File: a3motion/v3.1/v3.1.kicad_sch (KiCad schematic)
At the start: 0 parts

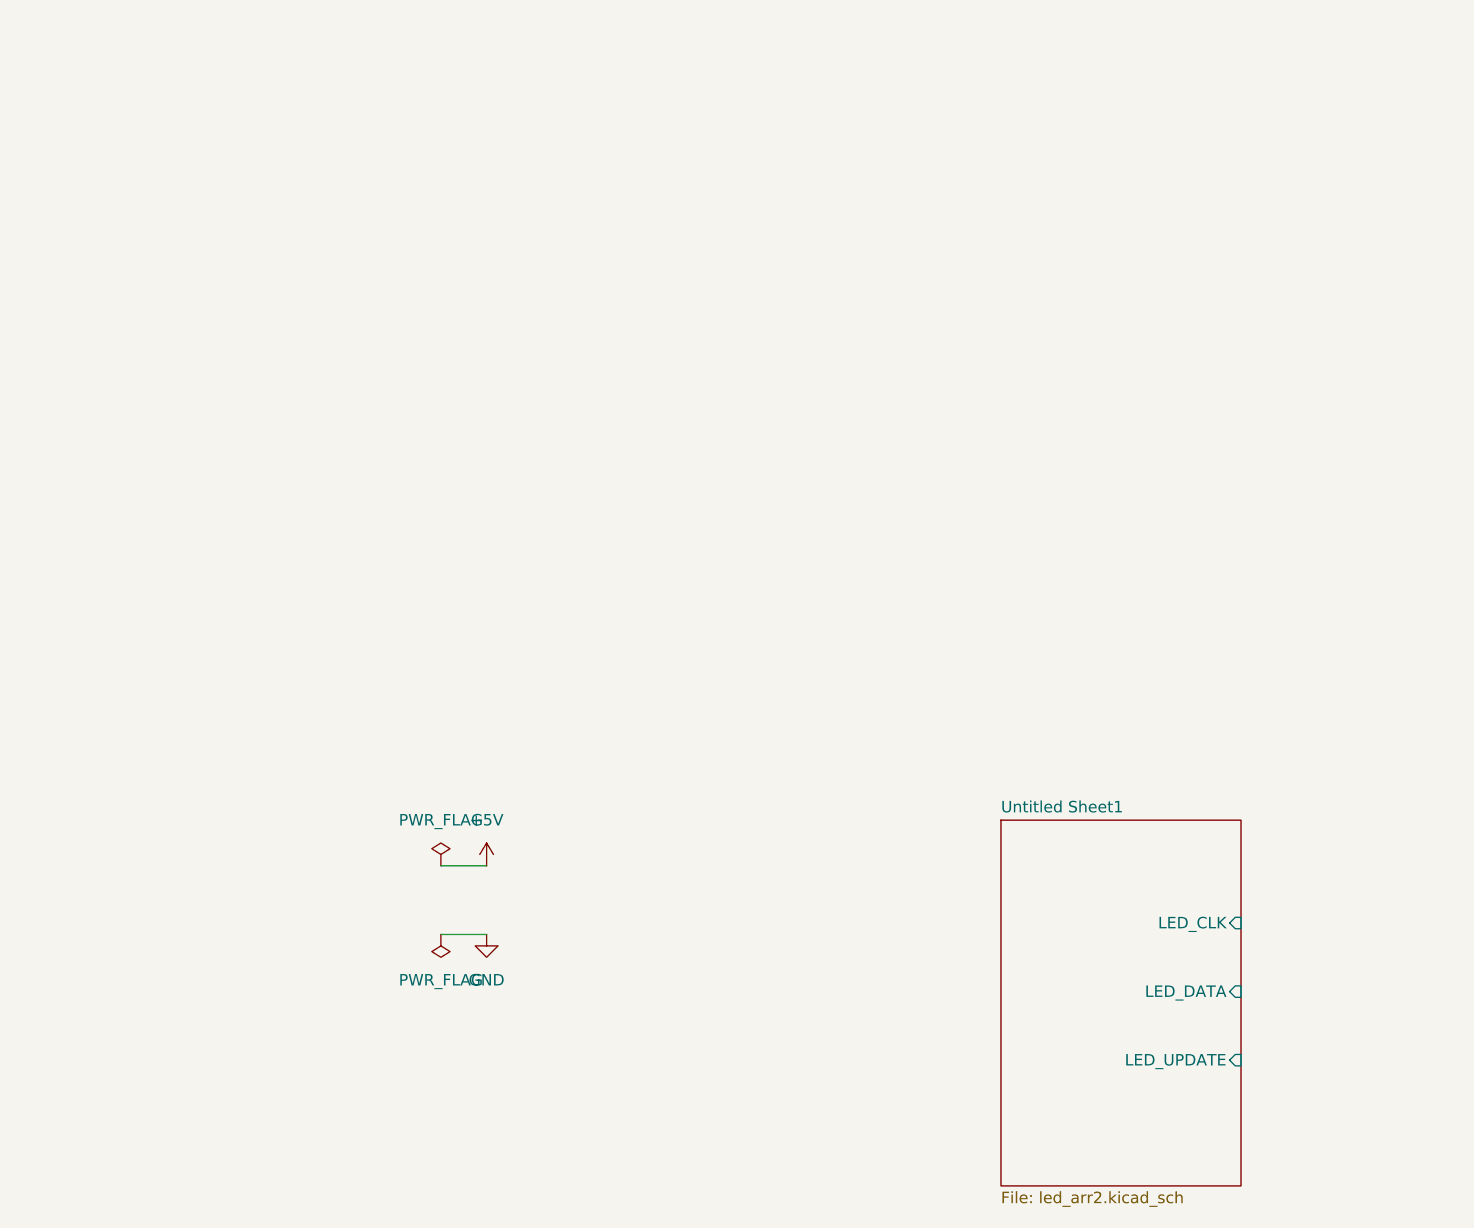
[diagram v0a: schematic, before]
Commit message: .
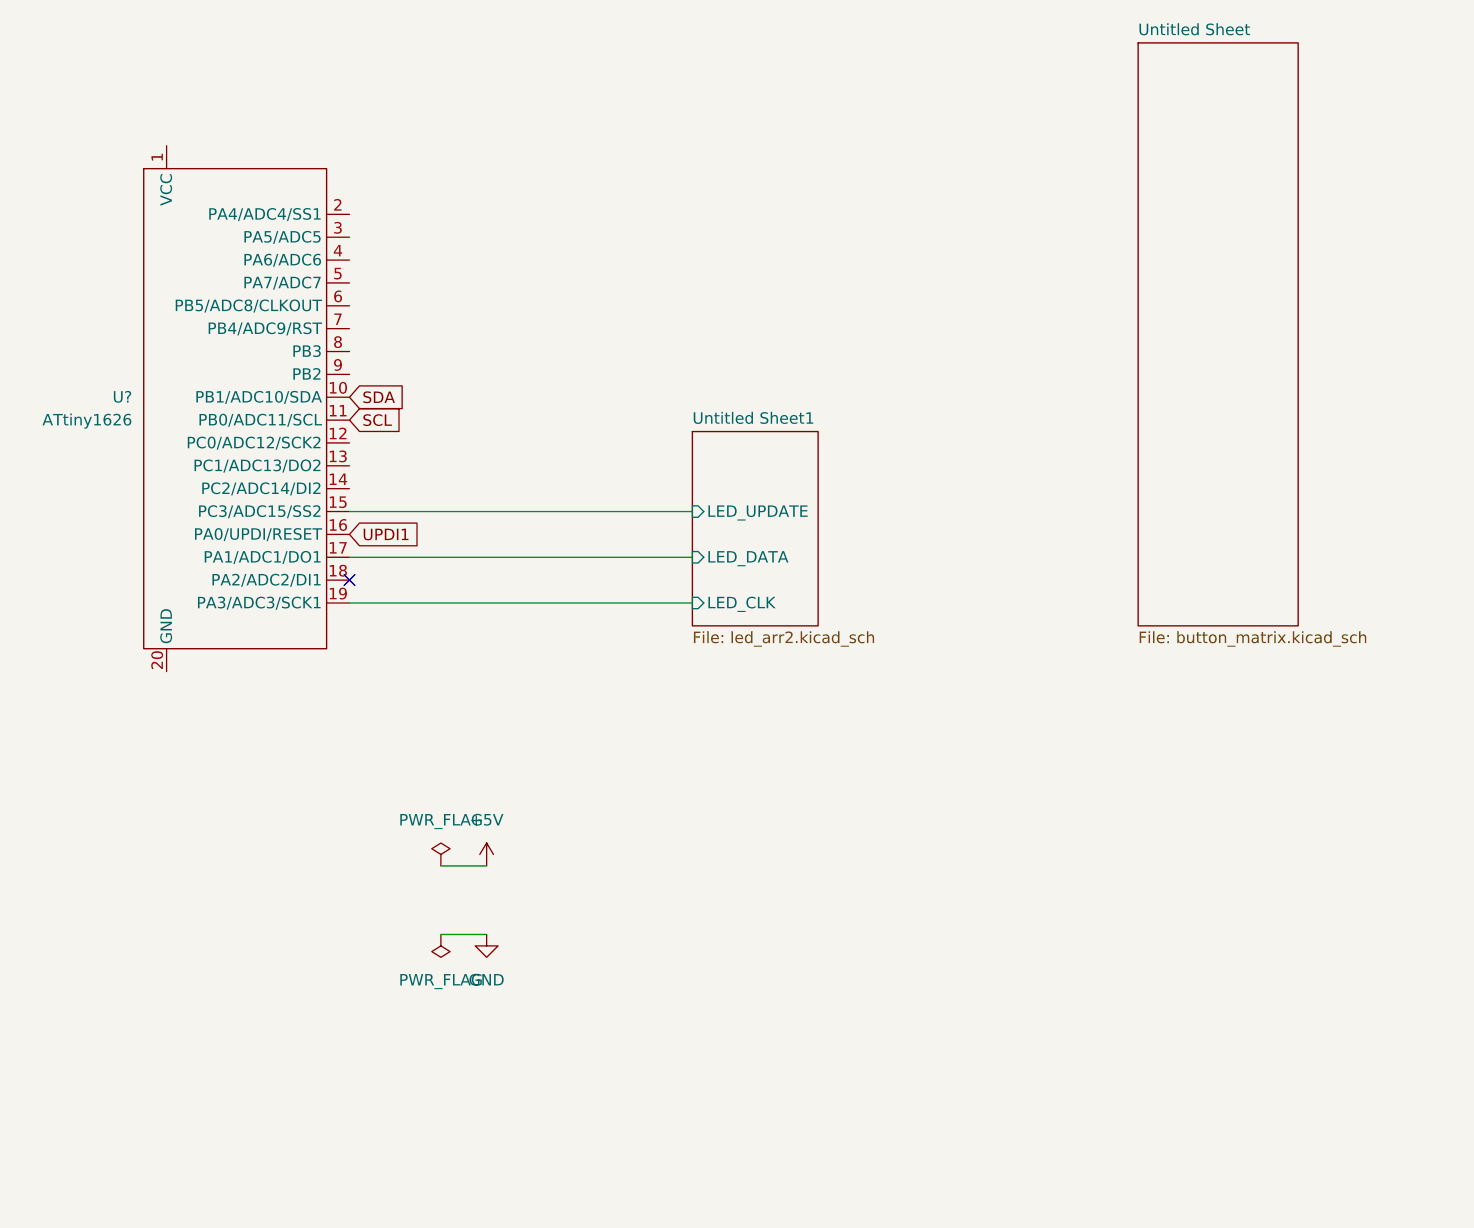
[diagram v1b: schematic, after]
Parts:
- added U?: ATtiny1626, attiny1626:SOIC127P1030X265-20N, symbol 3dAudioSym:ATtiny1626
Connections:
- net Untitled Sheet1/LED_CLK: now also U?.19 (PA3/ADC3/SCK1)
- net Untitled Sheet1/LED_DATA: now also U?.17 (PA1/ADC1/DO1)
- net Untitled Sheet1/LED_UPDATE: now also U?.15 (PC3/ADC15/SS2)
- new net SCL: U?.11 (PB0/ADC11/SCL)
- new net SDA: U?.10 (PB1/ADC10/SDA)
- new net UPDI1: U?.16 (PA0/UPDI/RESET)
- no-connect marks 0 -> 1
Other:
- added sheet Untitled Sheet (button_matrix.kicad_sch)
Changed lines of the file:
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@@
 (kicad_sch (version 20211123) (generator eeschema)
   (paper "A4")
+  (no_connect (at 53.34 82.55))
   (wire (pts (xy 63.5 114.3) (xy 68.58 114.3))
     (stroke (width 0) (type default) (color 0 0 0 0))
@@
   (wire (pts (xy 63.5 121.92) (xy 68.58 121.92))
     (stroke (width 0) (type default) (color 0 0 0 0))
+  )
+  (wire (pts (xy 53.34 80.01) (xy 91.44 80.01))
+    (stroke (width 0) (type default) (color 0 0 0 0))
+  )
+  (wire (pts (xy 53.34 74.93) (xy 91.44 74.93))
+    (stroke (width 0) (type default) (color 0 0 0 0))
+  )
+  (wire (pts (xy 53.34 85.09) (xy 91.44 85.09))
+    (stroke (width 0) (type default) (color 0 0 0 0))
+  )
+  (global_label "SCL" (shape input) (at 53.34 64.77 0) (fields_autoplaced)
+    (effects (font (size 1.27 1.27)) (justify left))
+    (property "Intersheet References" "${INTERSHEET_REFS}" (id 0) (at 59.2607 64.6906 0)
+      (effects (font (size 1.27 1.27)) (justify left) hide)
+    )
+  )
+  (global_label "UPDI1" (shape input) (at 53.34 77.47 0) (fields_autoplaced)
+    (effects (font (size 1.27 1.27)) (justify left))
+    (property "Intersheet References" "${INTERSHEET_REFS}" (id 0) (at 61.4379 77.3906 0)
+      (effects (font (size 1.27 1.27)) (justify left) hide)
+    )
+  )
+  (global_label "SDA" (shape input) (at 53.34 62.23 0) (fields_autoplaced)
+    (effects (font (size 1.27 1.27)) (justify left))
+    (property "Intersheet References" "${INTERSHEET_REFS}" (id 0) (at 59.3212 62.1506 0)
+      (effects (font (size 1.27 1.27)) (justify left) hide)
+    )
   )
   (symbol (lib_id "power:PWR_FLAG") (at 63.5 121.92 180) (unit 1)
@@
     (pin "1")
   )
-  (sheet (at 125.73 109.22) (size 26.67 40.64) (fields_autoplaced)
+  (symbol (lib_id "3dAudioSym:ATtiny1626") (at 41.91 64.77 0) (unit 1)
+    (in_bom yes) (on_board yes) (fields_autoplaced)
+    (property "Reference" "U?" (id 0) (at 29.21 62.2299 0)
+      (effects (font (size 1.27 1.27)) (justify right))
+    )
+    (property "Value" "ATtiny1626" (id 1) (at 29.21 64.7699 0)
+      (effects (font (size 1.27 1.27)) (justify right))
+    )
+    (property "Footprint" "attiny1626:SOIC127P1030X265-20N" (id 2) (at 53.34 39.37 0)
+      (effects (font (size 1.27 1.27)) hide)
+    )
+    (property "Datasheet" "" (id 3) (at 53.34 39.37 0)
+      (effects (font (size 1.27 1.27)) hide)
+    )
+    (pin "1")
+    (pin "10")
+    (pin "11")
+    (pin "12")
+    (pin "13")
+    (pin "14")
+    (pin "15")
+    (pin "16")
+    (pin "17")
+    (pin "18")
+    (pin "19")
+    (pin "2")
+    (pin "20")
+    (pin "3")
+    (pin "4")
+    (pin "5")
+    (pin "6")
+    (pin "7")
+    (pin "8")
+    (pin "9")
+  )
+  (sheet (at 91.44 66.04) (size 13.97 21.59) (fields_autoplaced)
     (stroke (width 0.1524) (type solid) (color 0 0 0 0))
     (fill (color 0 0 0 0.0000))
-    (property "Sheet name" "Untitled Sheet1" (id 0) (at 125.73 108.5084 0)
+    (property "Sheet name" "Untitled Sheet1" (id 0) (at 91.44 65.3284 0)
       (effects (font (size 1.27 1.27)) (justify left bottom))
     )
-    (property "Sheet file" "led_arr2.kicad_sch" (id 1) (at 125.73 150.4446 0)
+    (property "Sheet file" "led_arr2.kicad_sch" (id 1) (at 91.44 88.2146 0)
       (effects (font (size 1.27 1.27)) (justify left top))
     )
-    (pin "LED_CLK" input (at 152.4 120.65 0)
-      (effects (font (size 1.27 1.27)) (justify right))
-    )
-    (pin "LED_DATA" input (at 152.4 128.27 0)
-      (effects (font (size 1.27 1.27)) (justify right))
-    )
-    (pin "LED_UPDATE" input (at 152.4 135.89 0)
-      (effects (font (size 1.27 1.27)) (justify right))
+    (pin "LED_CLK" input (at 91.44 85.09 180)
+      (effects (font (size 1.27 1.27)) (justify left))
+    )
+    (pin "LED_DATA" input (at 91.44 80.01 180)
+      (effects (font (size 1.27 1.27)) (justify left))
+    )
+    (pin "LED_UPDATE" input (at 91.44 74.93 180)
+      (effects (font (size 1.27 1.27)) (justify left))
+    )
+  )
+  (sheet (at 140.97 22.86) (size 17.78 64.77) (fields_autoplaced)
+    (stroke (width 0.1524) (type solid) (color 0 0 0 0))
+    (fill (color 0 0 0 0.0000))
+    (property "Sheet name" "Untitled Sheet" (id 0) (at 140.97 22.1484 0)
+      (effects (font (size 1.27 1.27)) (justify left bottom))
+    )
+    (property "Sheet file" "button_matrix.kicad_sch" (id 1) (at 140.97 88.2146 0)
+      (effects (font (size 1.27 1.27)) (justify left top))
     )
   )
@@
     (path "/" (page "1"))
     (path "/8485fc92-3a6c-45d4-b117-a7f692d410d2" (page "3"))
+    (path "/fc444129-c0ee-4f1d-b15d-2ca12b630041" (page "3"))
   )
   (symbol_instances
@@
       (reference "R59") (unit 1) (value "4K7") (footprint "Resistor_SMD:R_1206_3216Metric_Pad1.30x1.75mm_HandSolder")
     )
+    (path "/fc444129-c0ee-4f1d-b15d-2ca12b630041/24e5708f-47e8-44cb-a8f1-6278ec5740e5"
+      (reference "R?") (unit 1) (value "R") (footprint "")
+    )
+    (path "/fc444129-c0ee-4f1d-b15d-2ca12b630041/3942fb96-a42e-455d-bf11-cb4cfc9b1fbd"
+      (reference "R?") (unit 1) (value "R") (footprint "")
+    )
+    (path "/fc444129-c0ee-4f1d-b15d-2ca12b630041/5a28c5f0-590c-4954-8ba8-3af237537b52"
+      (reference "R?") (unit 1) (value "R") (footprint "")
+    )
+    (path "/fc444129-c0ee-4f1d-b15d-2ca12b630041/5b3a3957-e2a8-4c0e-b421-5c753ea740f5"
+      (reference "R?") (unit 1) (value "R") (footprint "")
+    )
+    (path "/fc444129-c0ee-4f1d-b15d-2ca12b630041/635bd6f6-0714-4edd-8cc0-90ff7d08cab1"
+      (reference "R?") (unit 1) (value "R") (footprint "")
+    )
+    (path "/fc444129-c0ee-4f1d-b15d-2ca12b630041/88b0357f-5c8c-4fca-a7c2-9c8e643ff511"
+      (reference "R?") (unit 1) (value "R") (footprint "")
+    )
+    (path "/fc444129-c0ee-4f1d-b15d-2ca12b630041/a5884584-137e-4379-a7f7-6c3f1c075971"
+      (reference "R?") (unit 1) (value "R") (footprint "")
+    )
+    (path "/fc444129-c0ee-4f1d-b15d-2ca12b630041/d2182e5f-de5f-4505-85f8-51877d61a915"
+      (reference "R?") (unit 1) (value "R") (footprint "")
+    )
     (path "/8485fc92-3a6c-45d4-b117-a7f692d410d2/dcc539c5-e251-4449-af3b-095764ed56b3"
       (reference "U1") (unit 1) (value "TPIC6C595") (footprint "Package_SO:SOIC-16_3.9x9.9mm_P1.27mm")
@@
       (reference "U6") (unit 1) (value "TPIC6C595") (footprint "Package_SO:SOIC-16_3.9x9.9mm_P1.27mm")
     )
-  )
+    (path "/fc444129-c0ee-4f1d-b15d-2ca12b630041/1dc51fd4-c2fb-4171-8240-bdbc958c22ae"
+      (reference "U?") (unit 1) (value "touch_but_square") (footprint "3dAudioFoot:But_Velo_Rec_1")
+    )
+    (path "/fc444129-c0ee-4f1d-b15d-2ca12b630041/3e13a1a2-ca0d-42b0-b43f-ba376b17b285"
+      (reference "U?") (unit 1) (value "touch_but_square") (footprint "3dAudioFoot:But_Velo_Rec_1")
+    )
+    (path "/fc444129-c0ee-4f1d-b15d-2ca12b630041/45423905-ed29-4f70-9dcf-cd652ac5a9b5"
+      (reference "U?") (unit 1) (value "touch_but_square") (footprint "3dAudioFoot:But_Velo_Rec_1")
+    )
+    (path "/fc444129-c0ee-4f1d-b15d-2ca12b630041/4c65e03d-89f5-4300-9c87-d60c0ddf2549"
+      (reference "U?") (unit 1) (value "touch_but_square") (footprint "3dAudioFoot:But_Velo_Rec_1")
+    )
+    (path "/fc444129-c0ee-4f1d-b15d-2ca12b630041/7a1c3909-849a-4611-af6e-f3cb1ee24b93"
+      (reference "U?") (unit 1) (value "touch_but_square") (footprint "3dAudioFoot:But_Velo_Rec_1")
+    )
+    (path "/fc444129-c0ee-4f1d-b15d-2ca12b630041/83e1492b-c9b4-4514-9e11-54ef111e4f34"
+      (reference "U?") (unit 1) (value "BU4551BF-E2") (footprint "3dAudioFoot:SOIC127P620X171-16N")
+    )
+    (path "/fc444129-c0ee-4f1d-b15d-2ca12b630041/8d413166-5182-482b-bb07-bb4eba645a14"
+      (reference "U?") (unit 1) (value "touch_but_square") (footprint "3dAudioFoot:But_Velo_Rec_1")
+    )
+    (path "/fc444129-c0ee-4f1d-b15d-2ca12b630041/a3dc6ada-3c1e-4e5c-9cdb-19ce38eac1c0"
+      (reference "U?") (unit 1) (value "touch_but_square") (footprint "3dAudioFoot:But_Velo_Rec_1")
+    )
+    (path "/fc444129-c0ee-4f1d-b15d-2ca12b630041/ae1721ad-ac46-4923-b5e1-330ce0a12728"
+      (reference "U?") (unit 1) (value "touch_but_square") (footprint "3dAudioFoot:But_Velo_Rec_1")
+    )
+    (path "/b37f9070-5738-45a7-a012-b2901824103a"
+      (reference "U?") (unit 1) (value "ATtiny1626") (footprint "attiny1626:SOIC127P1030X265-20N")
+    )
+  )
